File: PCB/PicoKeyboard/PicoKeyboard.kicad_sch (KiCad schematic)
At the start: 5 parts, among them J1 USB_C_Receptacle_USB2.0_14P, J2 Conn_01x04_Socket, U1 Raspberry_Pi_Pico

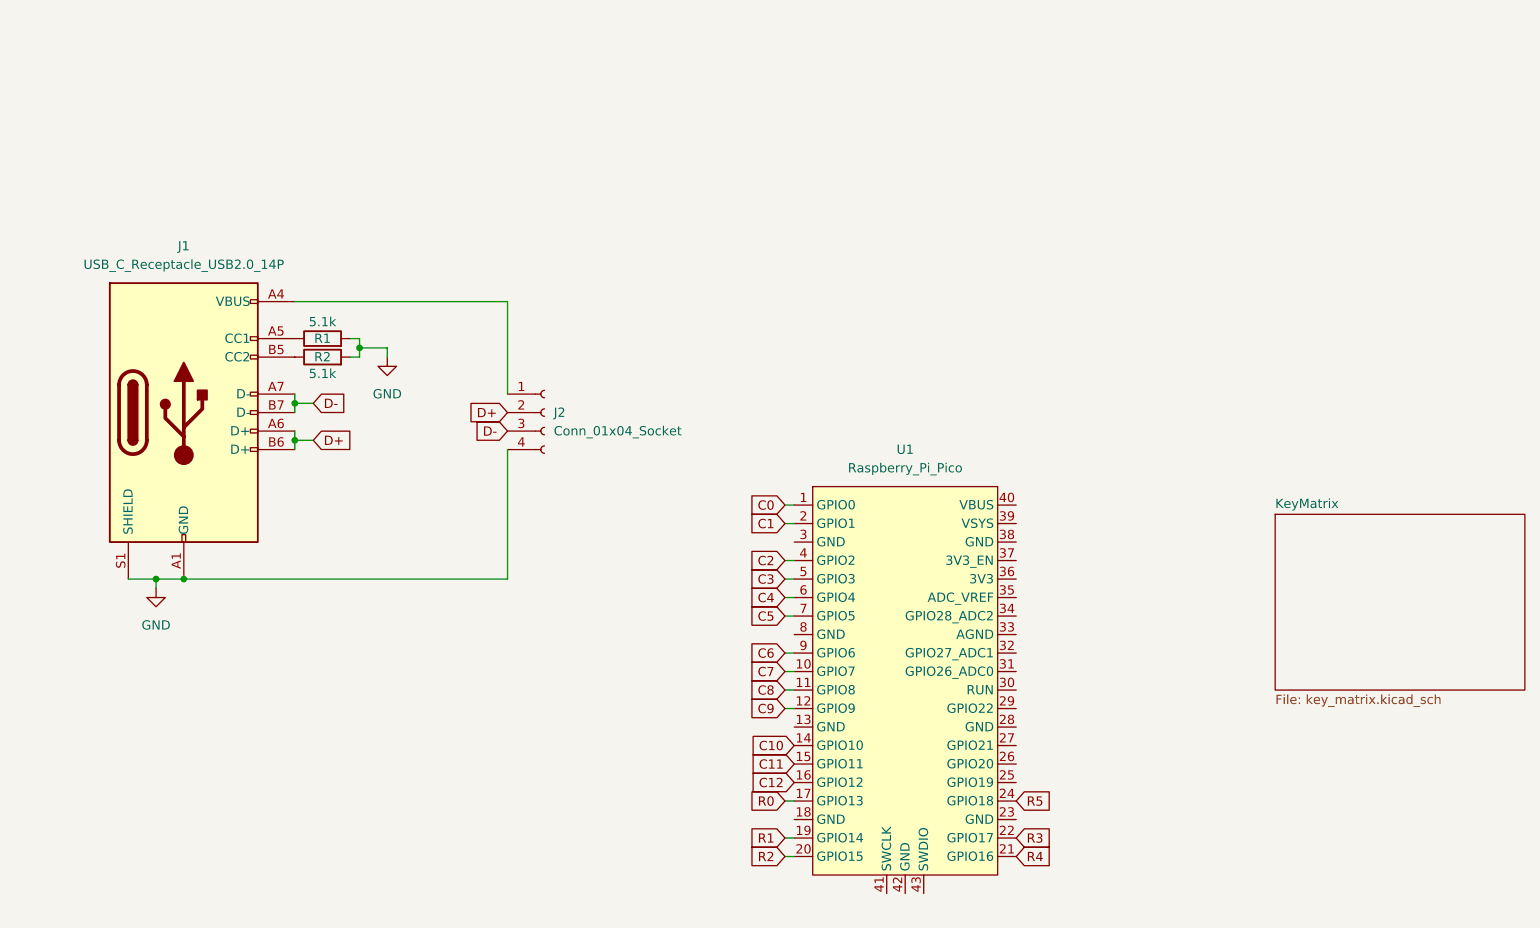
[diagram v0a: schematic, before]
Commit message: Fix
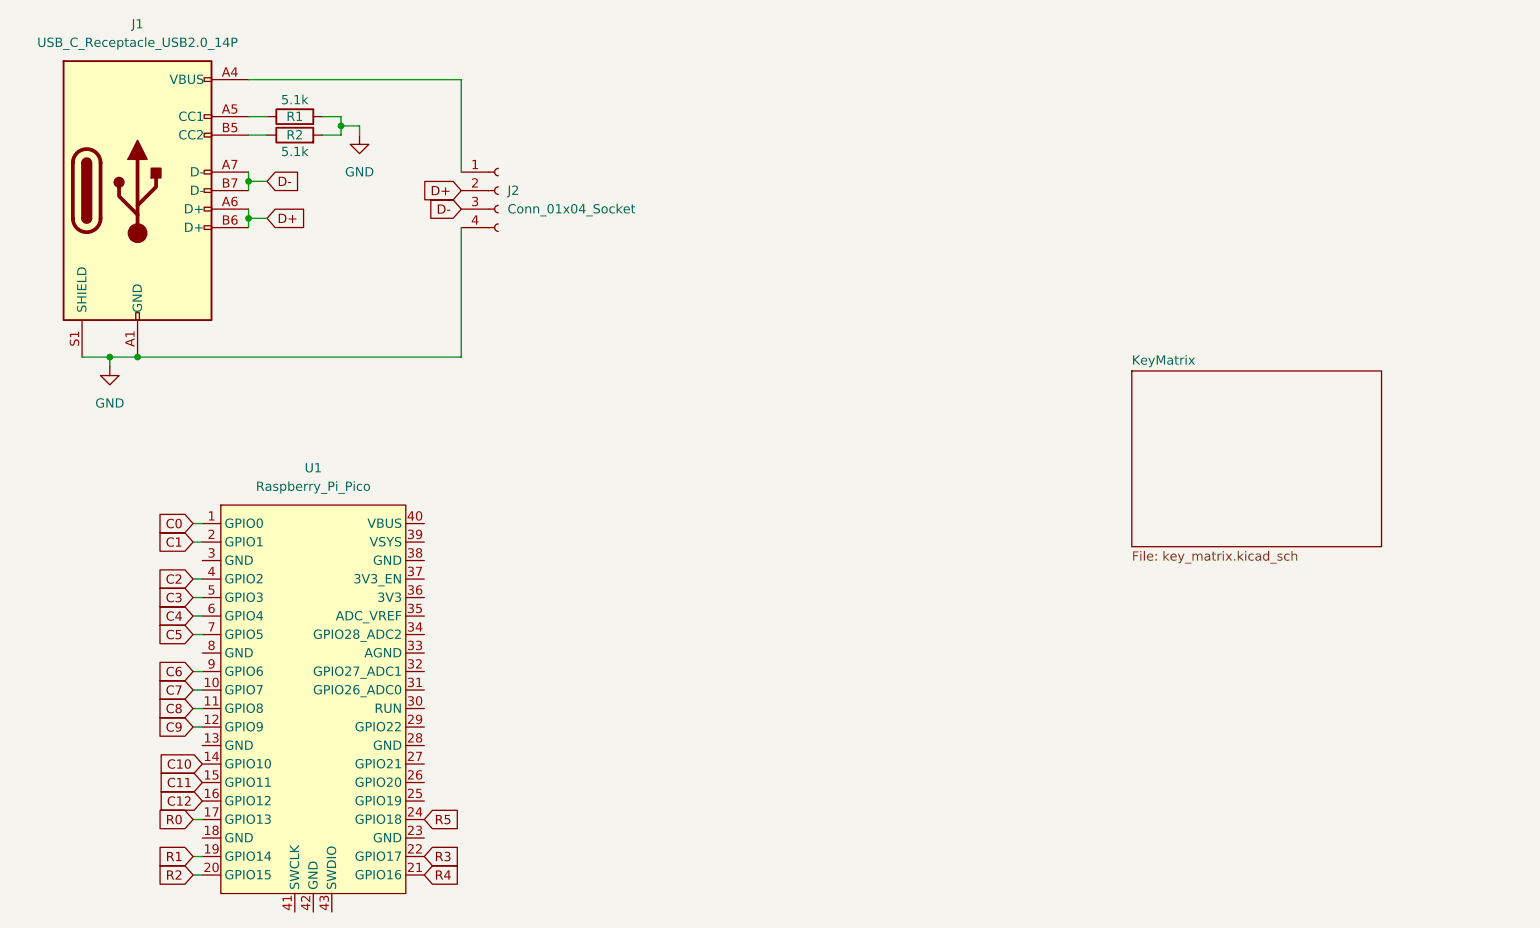
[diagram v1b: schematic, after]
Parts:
- R1, R2: footprint Resistor_SMD:R_0612_1632Metric_Pad1.18x3.40mm_HandSolder -> Resistor_SMD:R_0201_0603Metric_Pad0.64x0.40mm_HandSolder
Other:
- moved on the sheet: J1, J2, R1, R2, U1
